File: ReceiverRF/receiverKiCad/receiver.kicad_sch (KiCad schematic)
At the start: 23 parts, among them J2 Conn_01x05_Socket, U1 STM32F103RET6, Y1 CTX853CT-ND

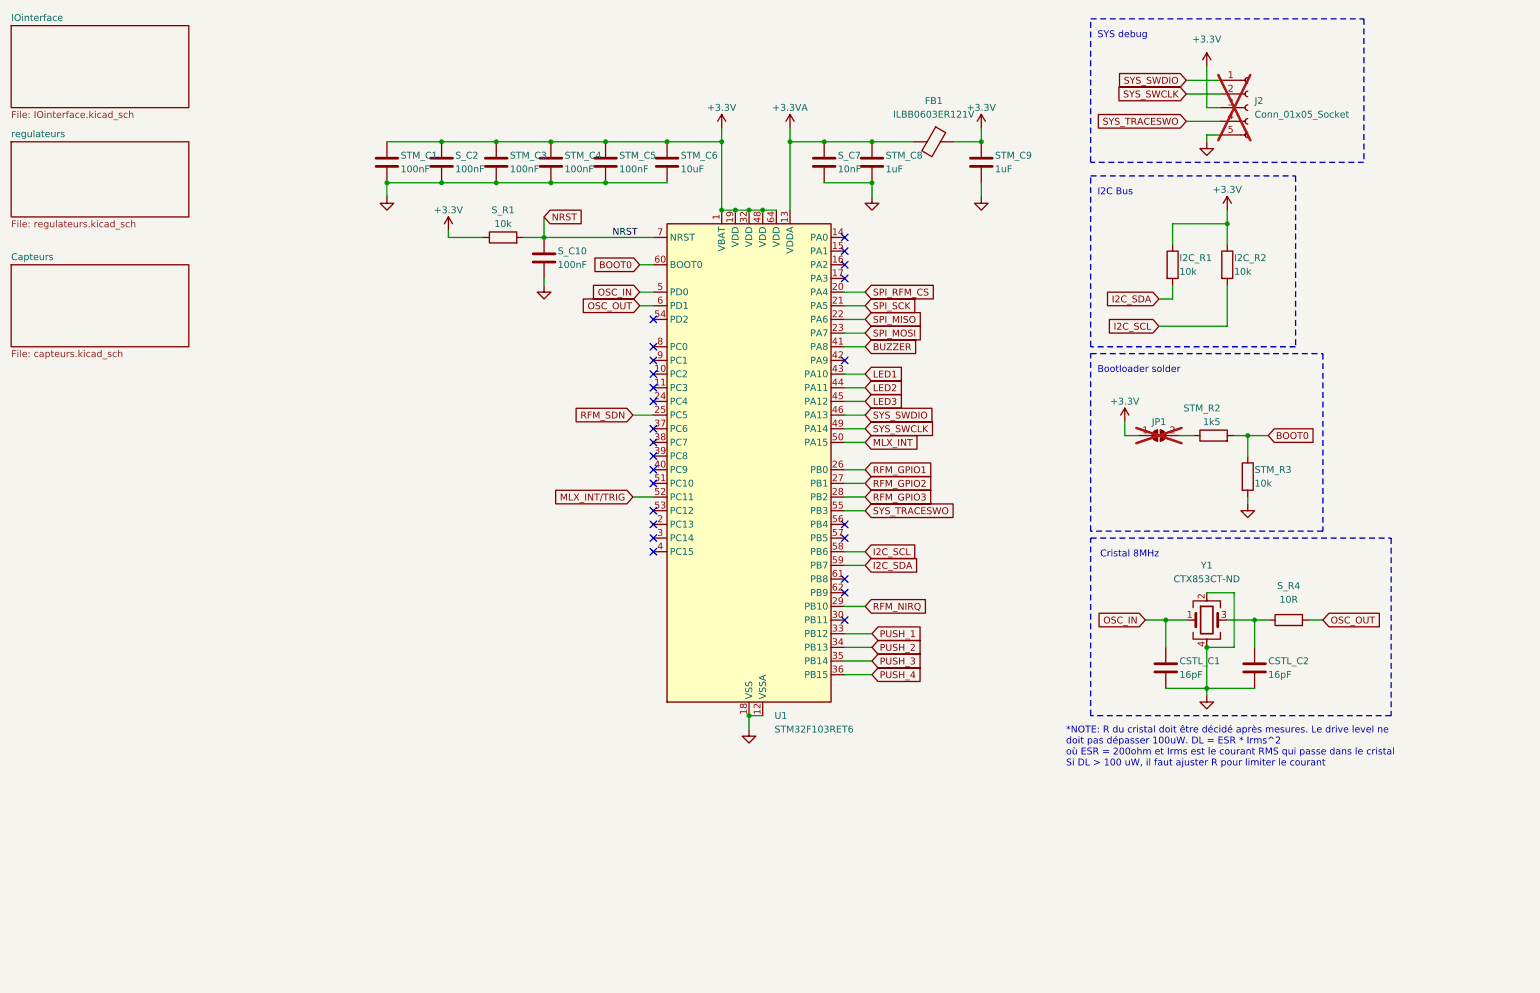
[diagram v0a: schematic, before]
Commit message: ideFIX v2 fix schematic, layout
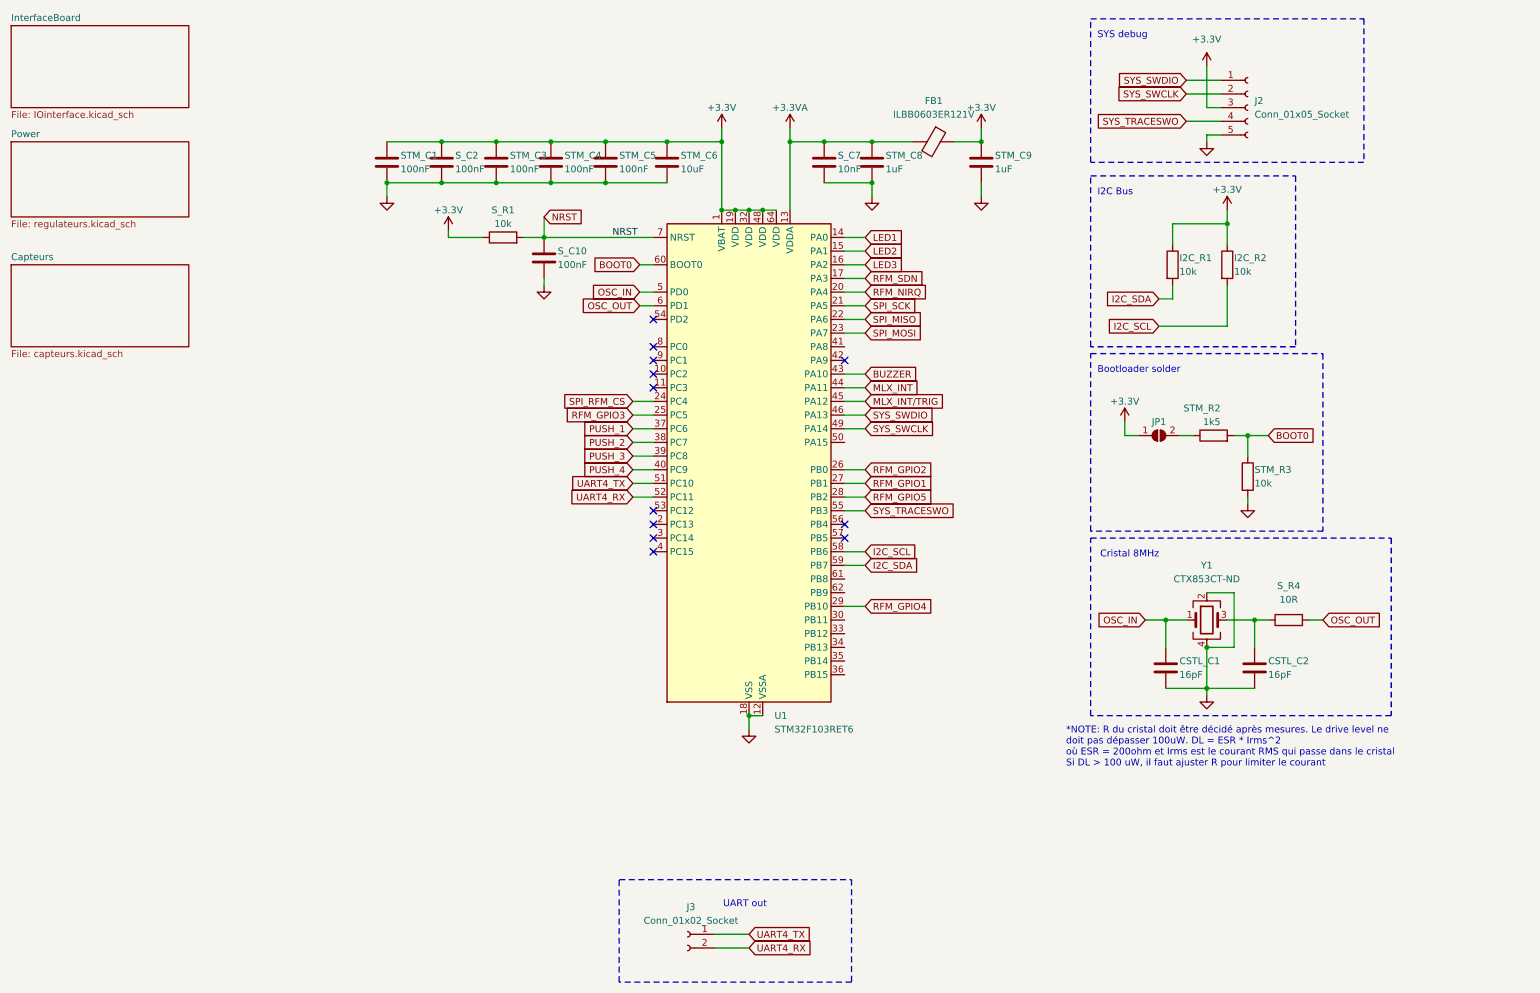
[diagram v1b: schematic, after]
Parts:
- added J3: Conn_01x02_Socket, Connector_PinHeader_2.54mm:PinHeader_1x02_P2.54mm_Vertical, symbol Connector:Conn_01x02_Socket
- J2: footprint Connector_PinHeader_2.00mm:PinHeader_1x05_P2.00mm_Vertical -> Connector_PinHeader_2.54mm:PinHeader_1x05_P2.54mm_Vertical; now fitted
- JP1: now fitted
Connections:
- net BUZZER: now also U1.43 (PA10); no longer U1.41 (PA8)
- net LED1: now also U1.14 (PA0); no longer U1.43 (PA10)
- net LED2: now also U1.15 (PA1); no longer U1.44 (PA11)
- net LED3: now also U1.16 (PA2); no longer U1.45 (PA12)
- net MLX_INT: now also U1.44 (PA11); no longer U1.50 (PA15)
- net MLX_INT/TRIG: now also U1.45 (PA12); no longer U1.52 (PC11)
- net PUSH_1: now also U1.37 (PC6); no longer U1.33 (PB12)
- net PUSH_2: now also U1.38 (PC7); no longer U1.34 (PB13)
- net PUSH_3: now also U1.39 (PC8); no longer U1.35 (PB14)
- net PUSH_4: now also U1.40 (PC9); no longer U1.36 (PB15)
- net RFM_GPIO1: now also U1.27 (PB1); no longer U1.26 (PB0)
- net RFM_GPIO2: now also U1.26 (PB0); no longer U1.27 (PB1)
- net RFM_GPIO3: now also U1.25 (PC5); no longer U1.28 (PB2)
- net RFM_NIRQ: now also U1.20 (PA4); no longer U1.29 (PB10)
- net RFM_SDN: now also U1.17 (PA3); no longer U1.25 (PC5)
- net SPI_RFM_CS: now also U1.24 (PC4); no longer U1.20 (PA4)
- net UART4_TX: now reaches U1.51 (PC10)
- net UART4_TX: now also J3.1 (Pin_1)
- new net RFM_GPIO4: U1.29 (PB10)
- new net RFM_GPIO5: U1.28 (PB2)
- new net UART4_RX: J3.2 (Pin_2), U1.52 (PC11)
- no-connect marks 25 -> 12
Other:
- sheet IOinterface renamed InterfaceBoard
- sheet regulateurs renamed Power
- note added: "UART out"
